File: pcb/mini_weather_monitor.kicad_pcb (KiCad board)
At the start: 2 copper layers, 135 x 72 mm, 12 parts, among them J1 SW-520D, U2 4.0inch_SPI_MSP4021, U2_BME280 module_bme280, U3_BH1750 module_bh1750

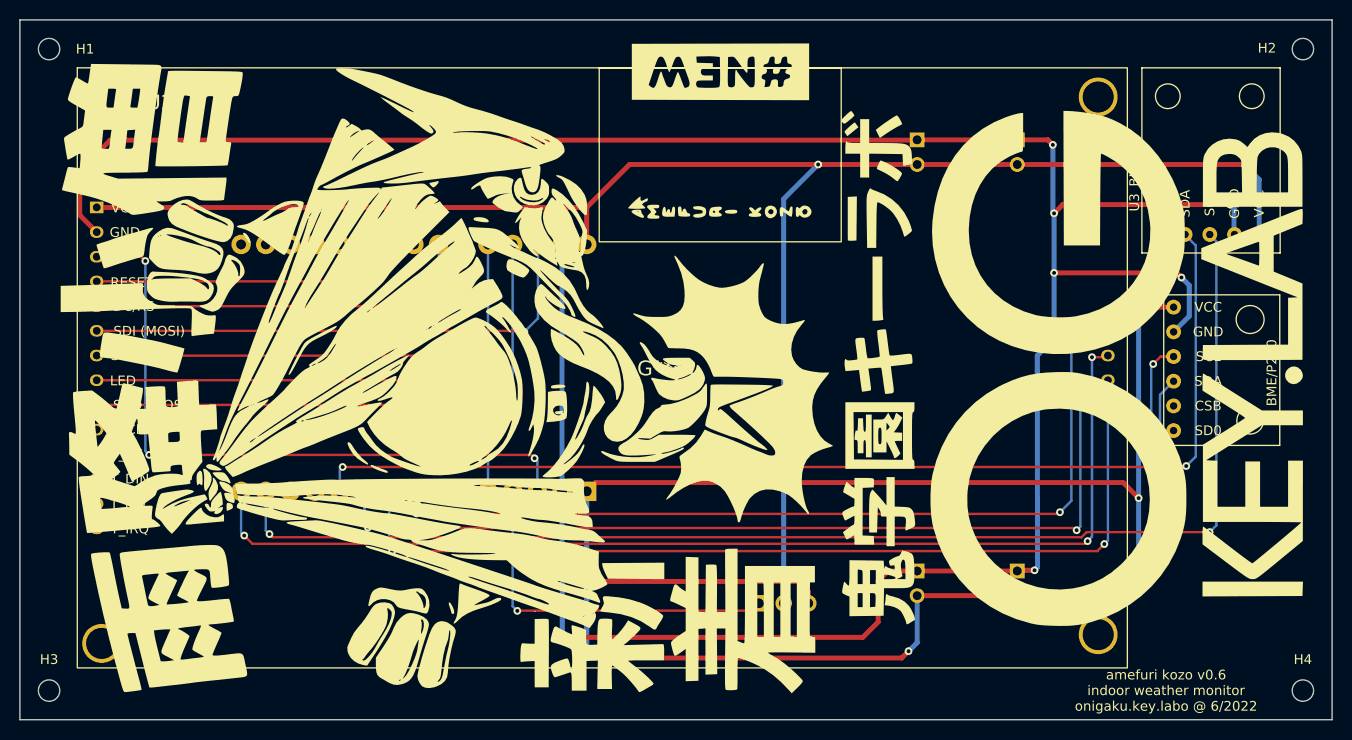
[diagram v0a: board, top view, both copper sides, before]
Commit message: revamping a bit
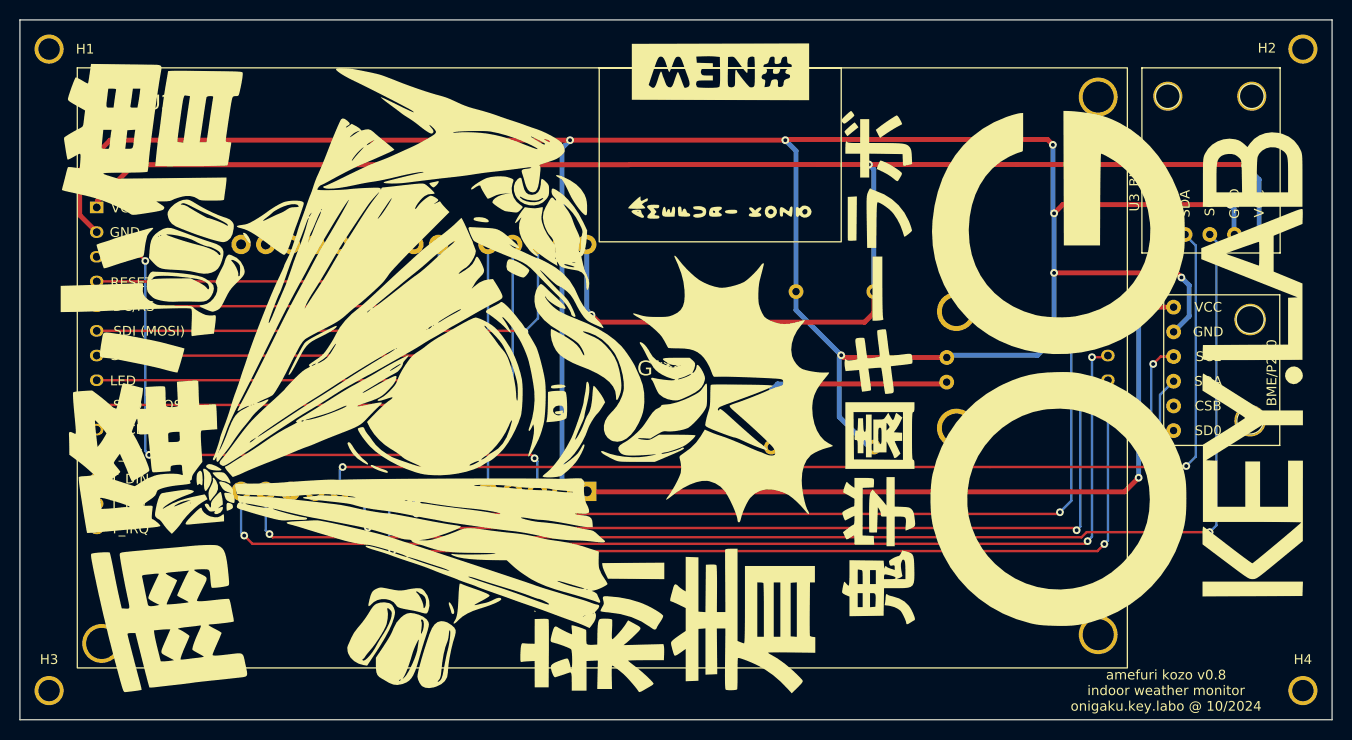
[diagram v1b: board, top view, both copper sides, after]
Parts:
- removed J1: SW-520D, tilt:KY020 Tilt
- removed Ue: PowerSupplyMB102_v13, power_supplies:POWERSUPPLYMB102
- added 5V_buck_boost1: ~, regulator_voltage:S09_HVN, B.Cu at (147.8, 100.5)
- added USB_C_Input1: ~, custom_usbc:USB_C_breakout_power_only, B.Cu at (160.2, 100.0)
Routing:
- net +3V3: track 169.0 -> 77.9 mm, vias 5 -> 2
- net GND: track 316.4 -> 265.4 mm
- net Net-(J1-Pin_1): track 37.7 -> 0.00 mm, vias 1 -> 0
- net VCC_PRE: track 0.00 -> 31.3 mm, vias 0 -> 1
- net VCC: track 178.4 -> 180.8 mm, vias 2 -> 3
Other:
- board text added: "amefuri kozo v0.8 indoor weather monitor onigaku.key.labo @ 10/2024"
- board text removed: "amefuri kozo v0.6 indoor weather monitor onigaku.key.labo @ 6/2022"
